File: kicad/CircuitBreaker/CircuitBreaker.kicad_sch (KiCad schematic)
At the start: 55 parts, among them J1 PH2.54, J4 PH2.54, J5 Conn_01x04_downlink, J6 Conn_01x04_uplink, J7 PH2.54, SW1 usbIAP, T1 CT104D, T2 CT104D, T3 CT104D, T4 CT104D, U1 LM324, U2 STC8H8K64U-45I-TSSOP20, U3 AP1117-33, U4 ESP-12E

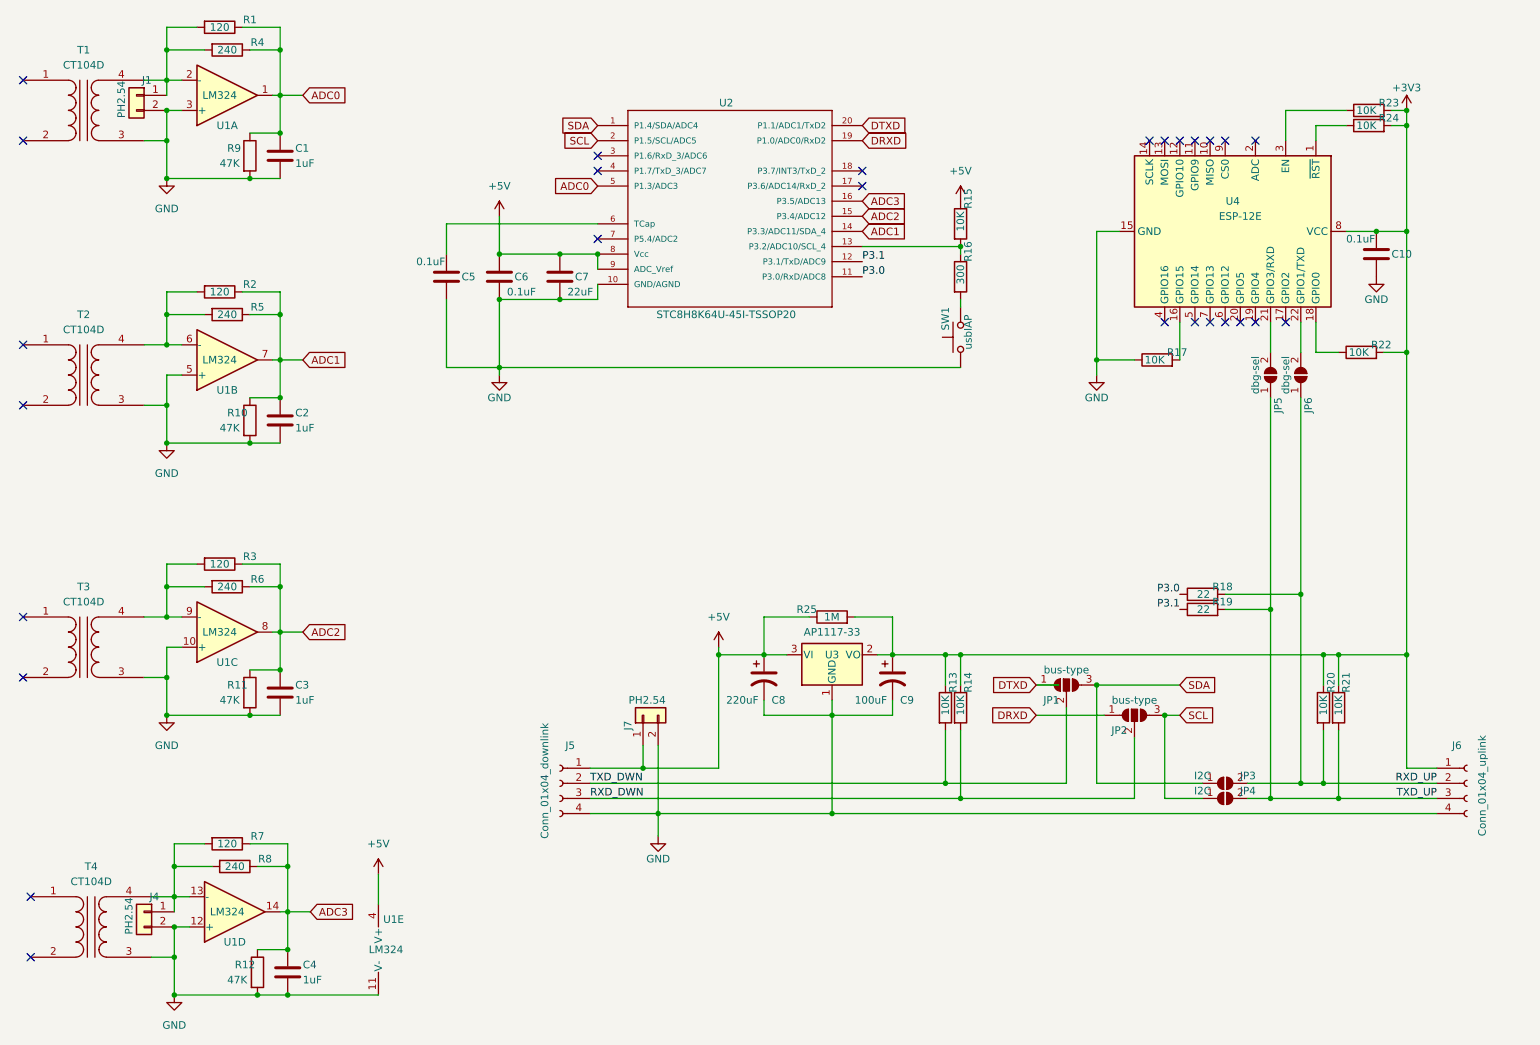
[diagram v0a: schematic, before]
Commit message: pcb rev
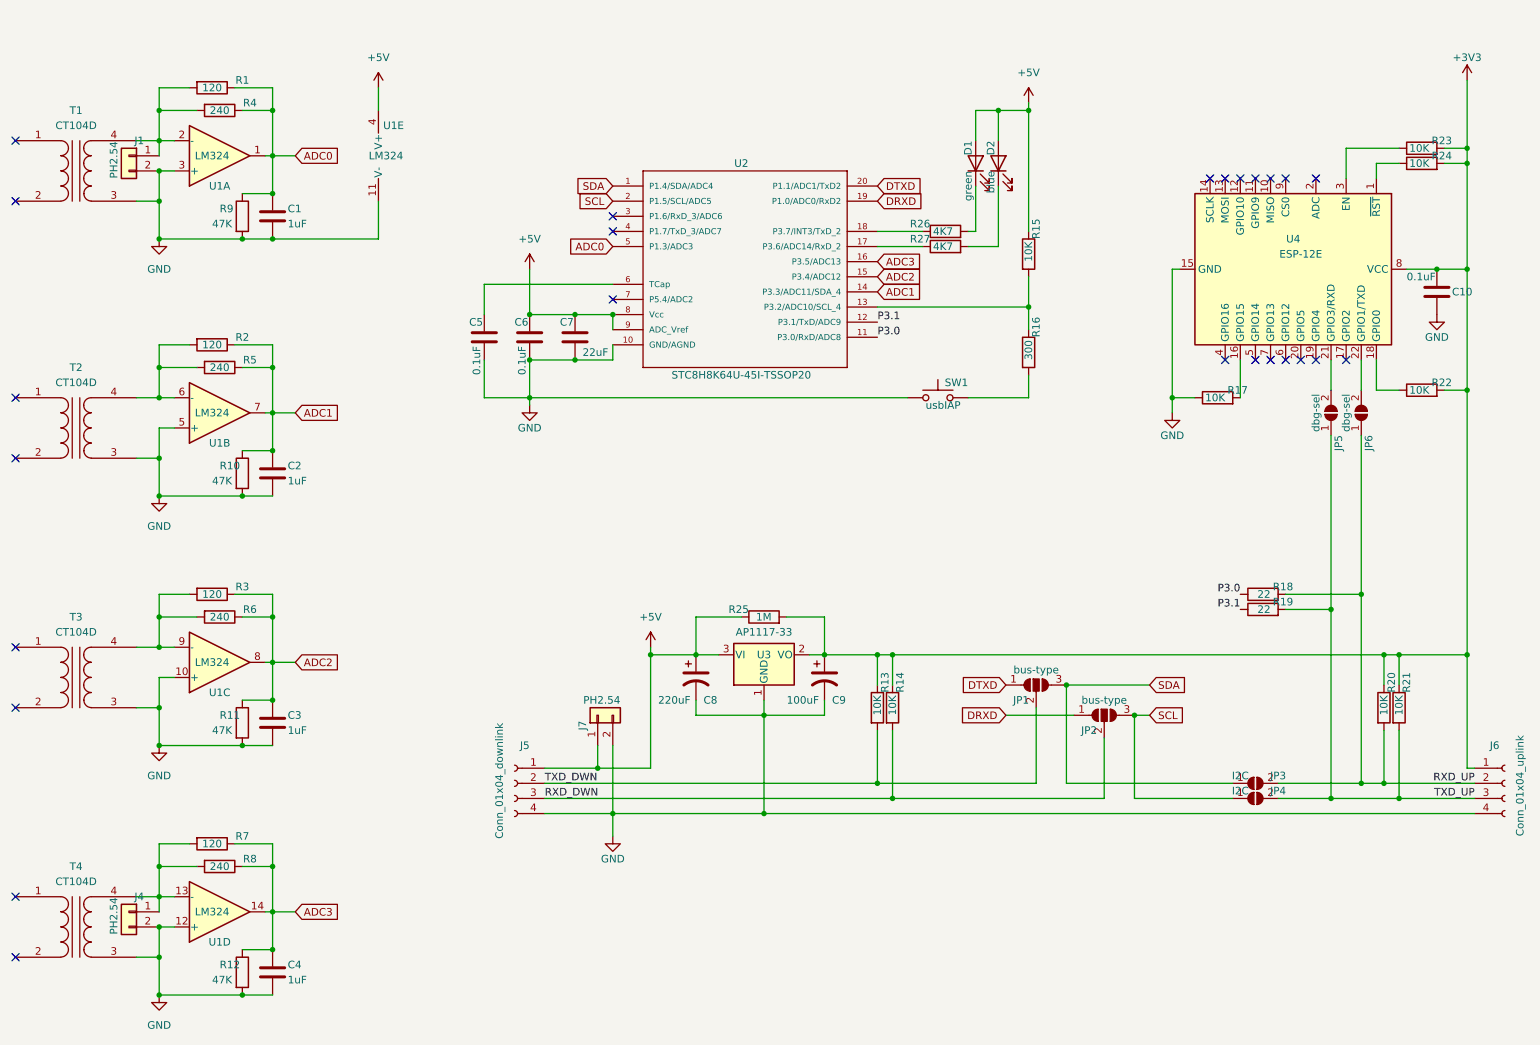
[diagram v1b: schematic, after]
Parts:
- added D1: green, LED_SMD:LED_0603_1608Metric, symbol Device:LED
- added D2: blue, LED_SMD:LED_0603_1608Metric, symbol Device:LED
- added R26, R27: 4K7, Resistor_SMD:R_0603_1608Metric, symbol Device:R
- JP5, JP6: footprint Jumper:SolderJumper-2_P1.3mm_Open_RoundedPad1.0x1.5mm -> Jumper:SolderJumper-2_P1.3mm_Bridged_RoundedPad1.0x1.5mm
- R1, R2, R3, R7: footprint Resistor_THT:R_Axial_DIN0204_L3.6mm_D1.6mm_P1.90mm_Vertical -> Resistor_THT:R_Axial_DIN0204_L3.6mm_D1.6mm_P7.62mm_Horizontal
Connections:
- net +5V: now also D1.2 (A), D2.2 (A)
- net at U2.17 (P3.6/ADC14/RxD_2): now also R27.1
- net at U2.18 (P3.7/INT3/TxD_2): now also R26.1
- new net: D2.1 (K), R27.2
- new net: D1.1 (K), R26.2
- no-connect marks 27 -> 25
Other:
- moved on the sheet: C1, C10, C2, C3, C4, C5, C6, C7, C8, C9, J1, J4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
